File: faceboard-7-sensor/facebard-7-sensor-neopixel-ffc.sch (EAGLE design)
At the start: 38 parts, among them Q1 QRE1113, Q2 QRE1113, Q3 QRE1113, Q4 QRE1113, Q5 QRE1113, Q6 QRE1113, Q7 QRE1113, U1 CD4051BE

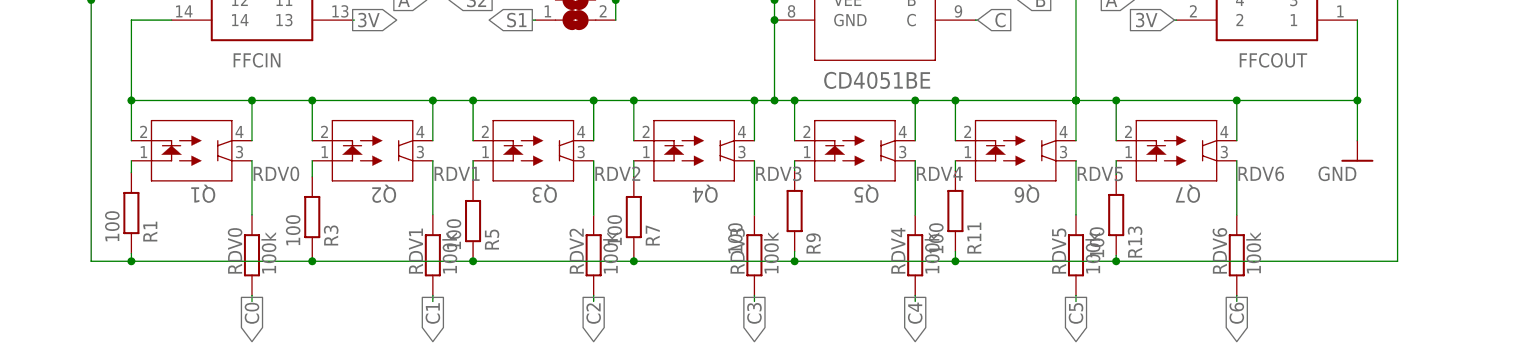
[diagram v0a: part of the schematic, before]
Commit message: fix signal routing
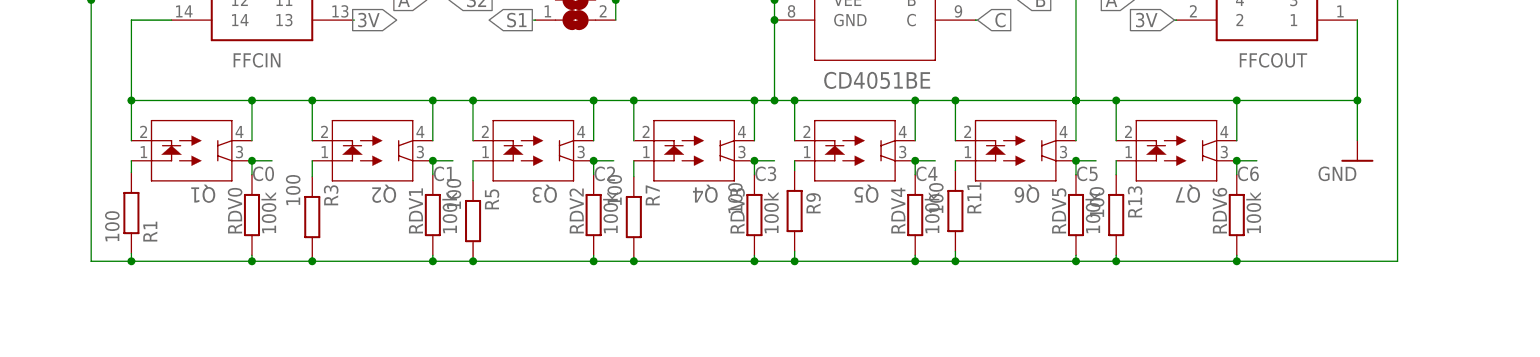
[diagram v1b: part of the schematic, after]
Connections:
- removed net RDV0: Q1.3, RDV0.2
- removed net RDV1: Q2.3, RDV1.2
- removed net RDV2: Q3.3, RDV2.2
- removed net RDV3: Q4.3, RDV3.2
- removed net RDV4: Q5.3, RDV4.2
- removed net RDV5: Q6.3, RDV5.2
- removed net RDV6: Q7.3, RDV6.2
- net 5V: now also RDV0.1, RDV1.1, RDV2.1, RDV3.1, RDV4.1, RDV5.1, RDV6.1
- net C0: now also Q1.3, RDV0.2; no longer RDV0.1
- net C1: now also Q2.3, RDV1.2; no longer RDV1.1
- net C2: now also Q3.3, RDV2.2; no longer RDV2.1
- net C3: now also Q4.3, RDV3.2; no longer RDV3.1
- net C4: now also Q5.3, RDV4.2; no longer RDV4.1
- net C5: now also Q6.3, RDV5.2; no longer RDV5.1
- net C6: now also Q7.3, RDV6.2; no longer RDV6.1
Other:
- moved on the sheet: RDV0, RDV1, RDV2, RDV3, RDV4, RDV5, RDV6
